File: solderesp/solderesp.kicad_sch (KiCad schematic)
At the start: 2 parts, among them U1 ESP32-WROOM-32

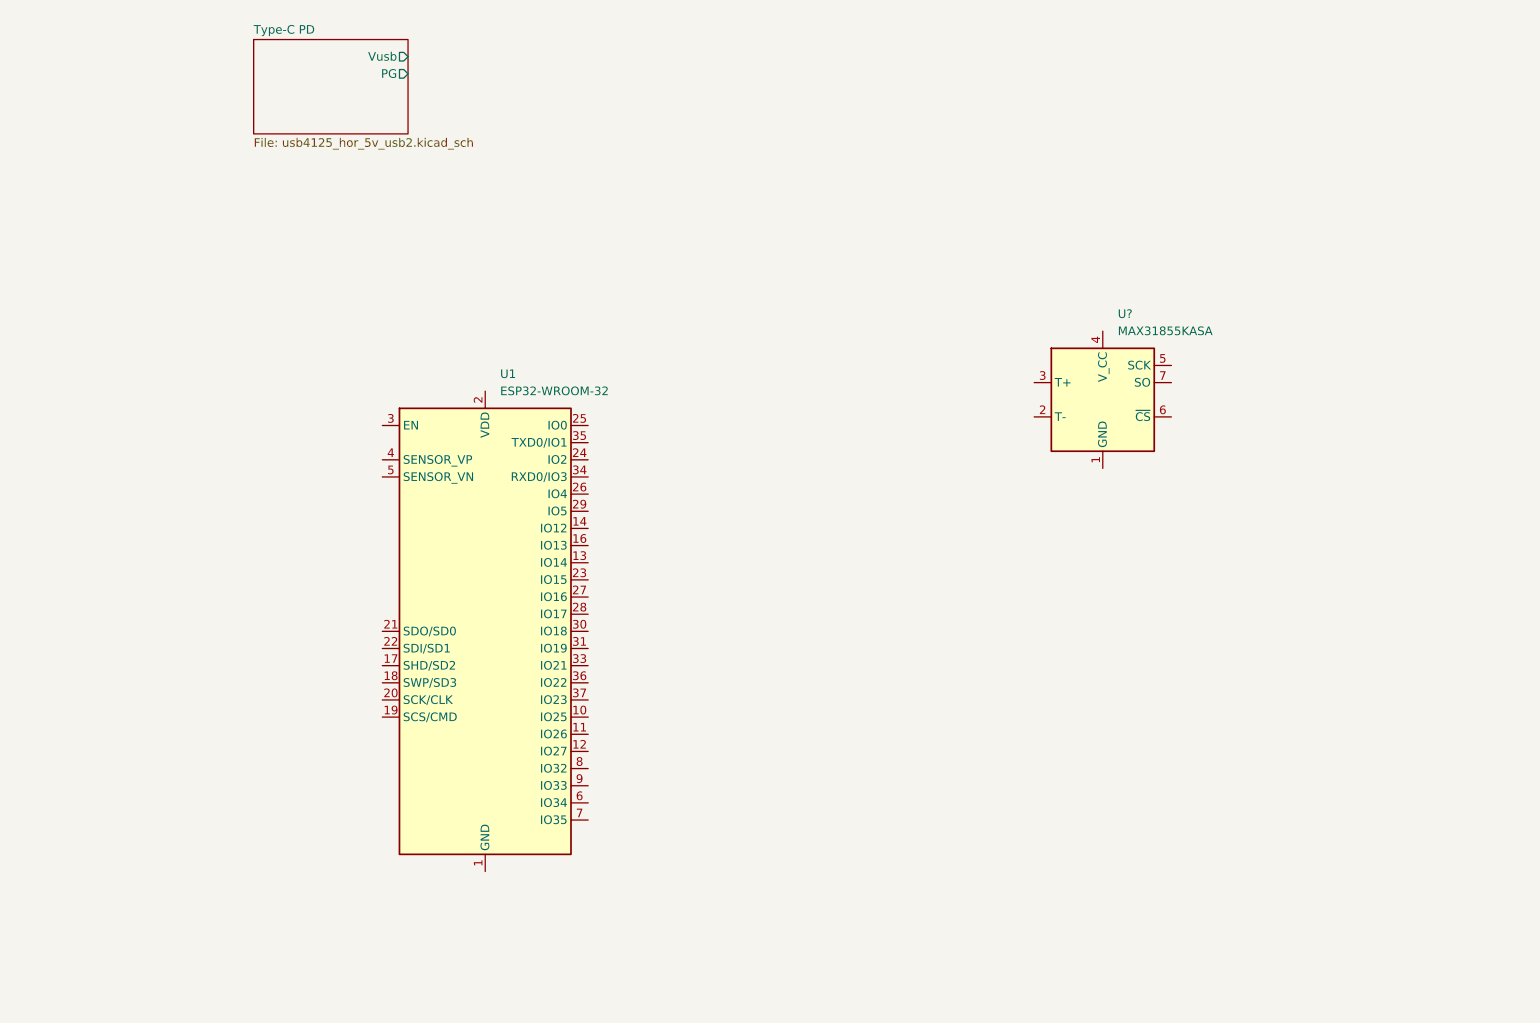
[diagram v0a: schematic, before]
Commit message: Required symbols SCH & 3D has been added
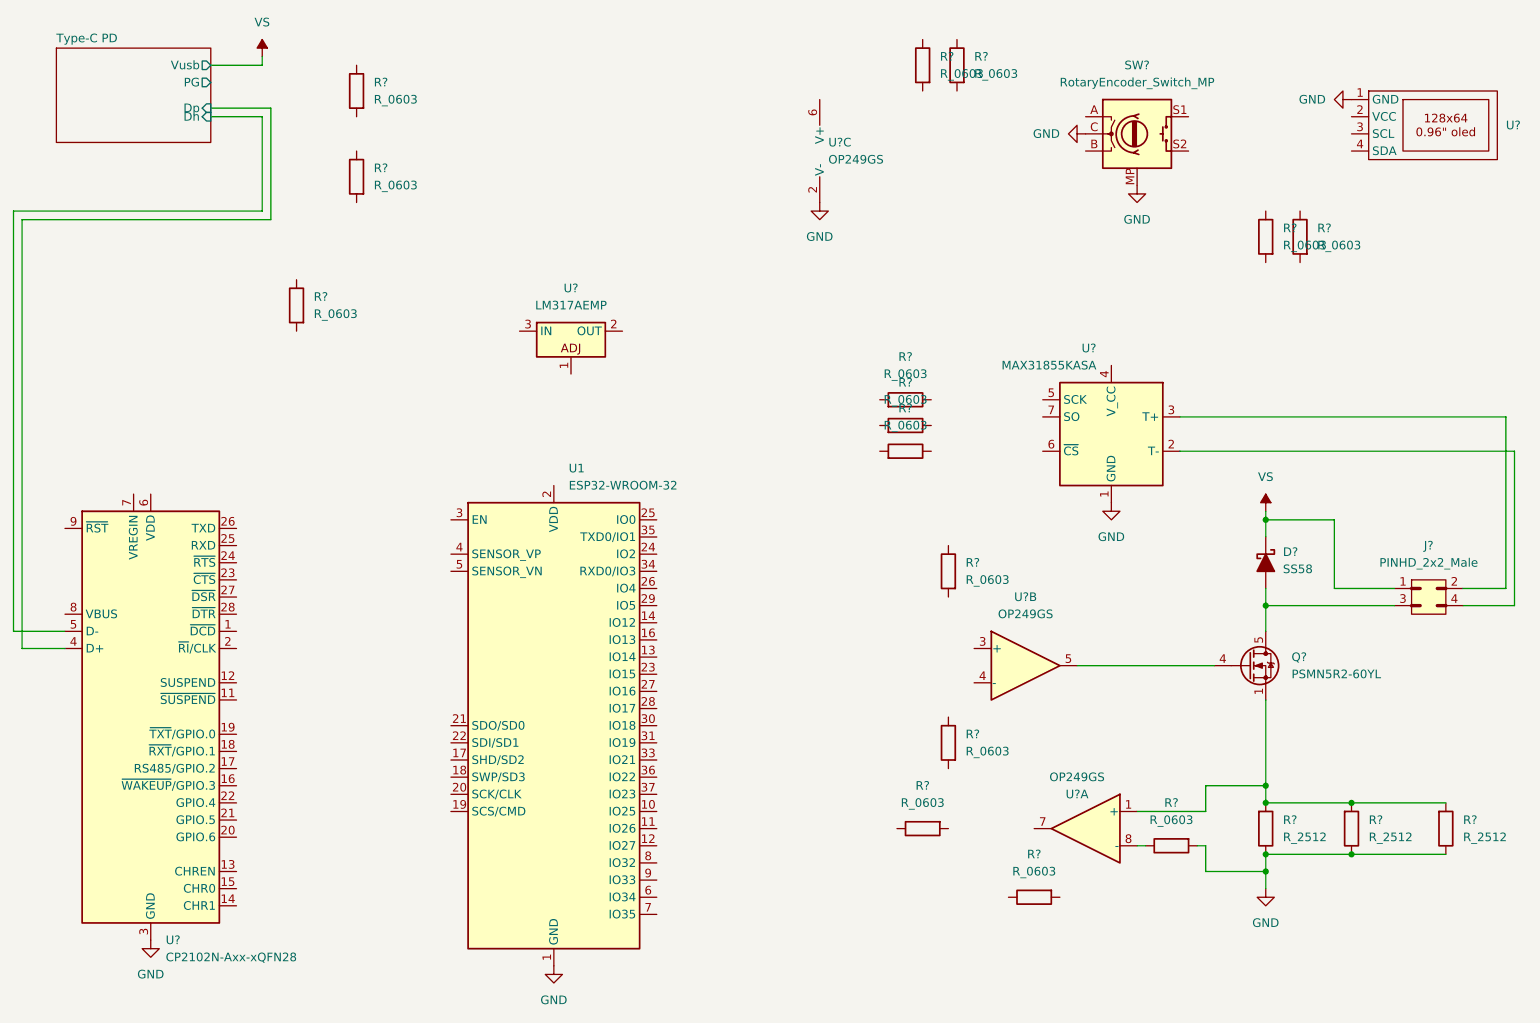
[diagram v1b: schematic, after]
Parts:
- added D?: SS58, PCM_Diode_SMD_AKL:D_SMC, symbol PCM_Diode_Schottky_AKL:SS58
- added J?: PINHD_2x2_Male, Connector_PinHeader_2.54mm:PinHeader_2x02_P2.54mm_Vertical, symbol PCM_SL_Pin_Headers:PINHD_2x2_Male
- added Q?: PSMN5R2-60YL, Package_TO_SOT_SMD:LFPAK56, symbol Transistor_FET:PSMN5R2-60YL
- added R? (x15): R_0603, PCM_Resistor_SMD_AKL:R_0603_1608Metric, symbol PCM_Resistor_AKL:R_0603
- added R? (x3): R_2512, PCM_Resistor_SMD_AKL:R_2512_6332Metric, symbol PCM_Resistor_AKL:R_2512
- added SW?: RotaryEncoder_Switch_MP, symbol Device:RotaryEncoder_Switch_MP
- added U? (x3): OP249GS, Package_SO:SOIC-8_3.9x4.9mm_P1.27mm, symbol Amplifier_Operational:OP249GS
- added U?: LM317AEMP, PCM_Package_TO_SOT_SMD_AKL:SOT-223-3_TabPin2, symbol PCM_Voltage_Regulator_AKL:LM317AEMP
- added U?: ~, symbol solder_sym:oled_ssd1306_128x64
- added U?: CP2102N-Axx-xQFN28, Package_DFN_QFN:QFN-28-1EP_5x5mm_P0.5mm_EP3.35x3.35mm, symbol Interface_USB:CP2102N-Axx-xQFN28
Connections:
- net GND: now reaches U?.1 (GND)
- net GND: now also U1.1 (GND), U1.15 (GND), U1.38 (GND), U1.39 (GND), R?.1, R?.2, R?.2, R?.2, SW?.C, SW?.MP, U?.1 (GND), U?.2 (V-), U?.29 (GND), U?.3 (GND)
- net at U?.2 (T-): now also J?.4
- net at U?.3 (T+): now also J?.2
- new net: Q?.4 (G), U?.5
- new net: D?.2 (A), J?.3, Q?.5 (D)
- new net: Q?.1 (S), Q?.2 (S), Q?.3 (S), R?.1, R?.1, R?.1, U?.1 (+)
- new net: R?.2, U?.8 (-)
- new net Type-C PD/Dn: U?.5 (D-)
- new net Type-C PD/Dp: U?.4 (D+)
- new net VS: D?.1 (K), J?.1
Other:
- sheet Type-C PD ports: added Dn, Dp; removed none
- moved on the sheet: U1, U?
